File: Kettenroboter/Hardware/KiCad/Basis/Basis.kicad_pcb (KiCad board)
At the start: 2 copper layers, 90.6 x 101.2 mm, 106 parts, among them J1 691103110002, J10 691103110002, J11 Conn_01x03, J12 Conn_01x03, J13 Conn_01x03, J14 Conn_01x03, J15 Conn_01x01, J16 Conn_01x03, J17 Conn_01x03, J18 691103110002, J19 691103110002, J2 691103110002, J20 691103110002, J21 691103110002, J22 691103110002, J23 691103110002, J24 691103110002, J25 691103110002, J26 691103110002, J27 691103110002, J28 Conn_01x02, J3 691103110002, J4 691103110002, J5 691103110002, J6 691103110002, J7 691103110002, J8 691103110002, J9 691103110002, Q1 BSS138, Q2 BSS138, Q3 BSS138, Q4 BSS138, Q5 NMOS, Q6 NMOS, U2 NCP1117LPST33T3G, U3 SN74LS07

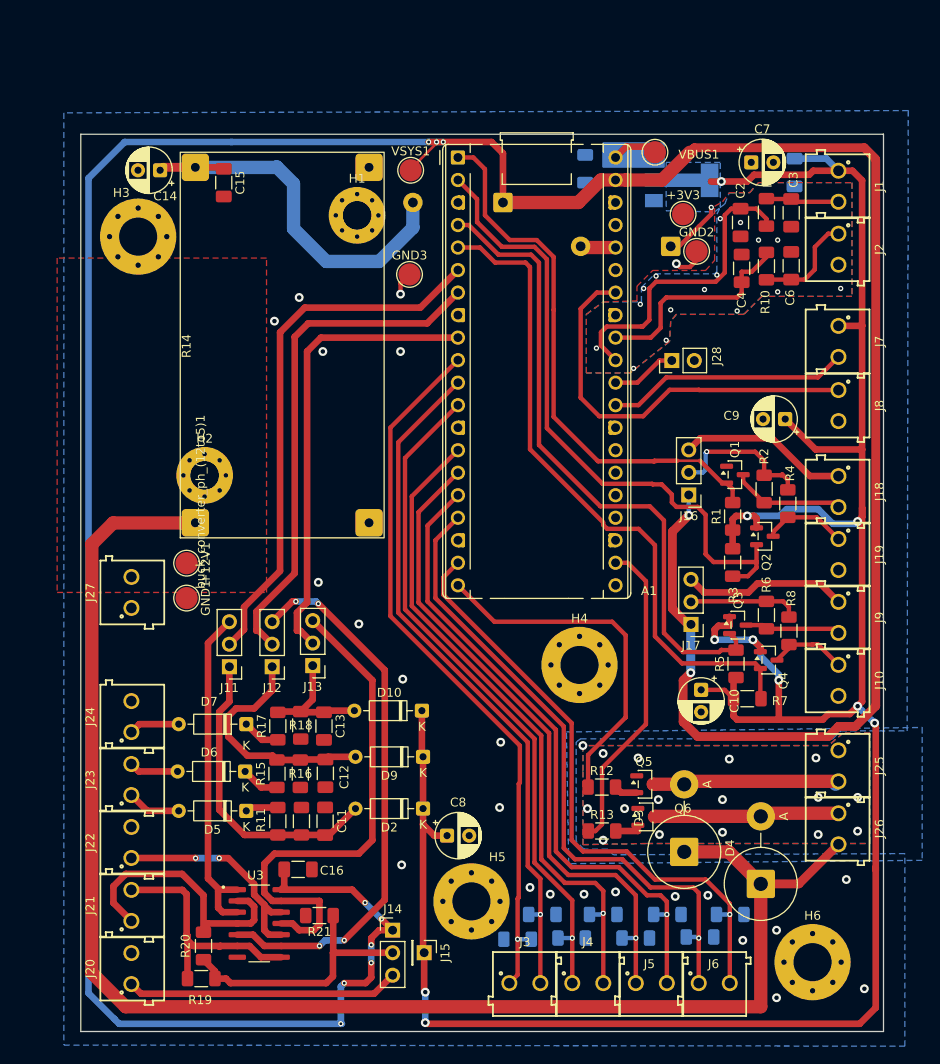
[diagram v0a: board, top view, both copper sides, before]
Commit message: final final final
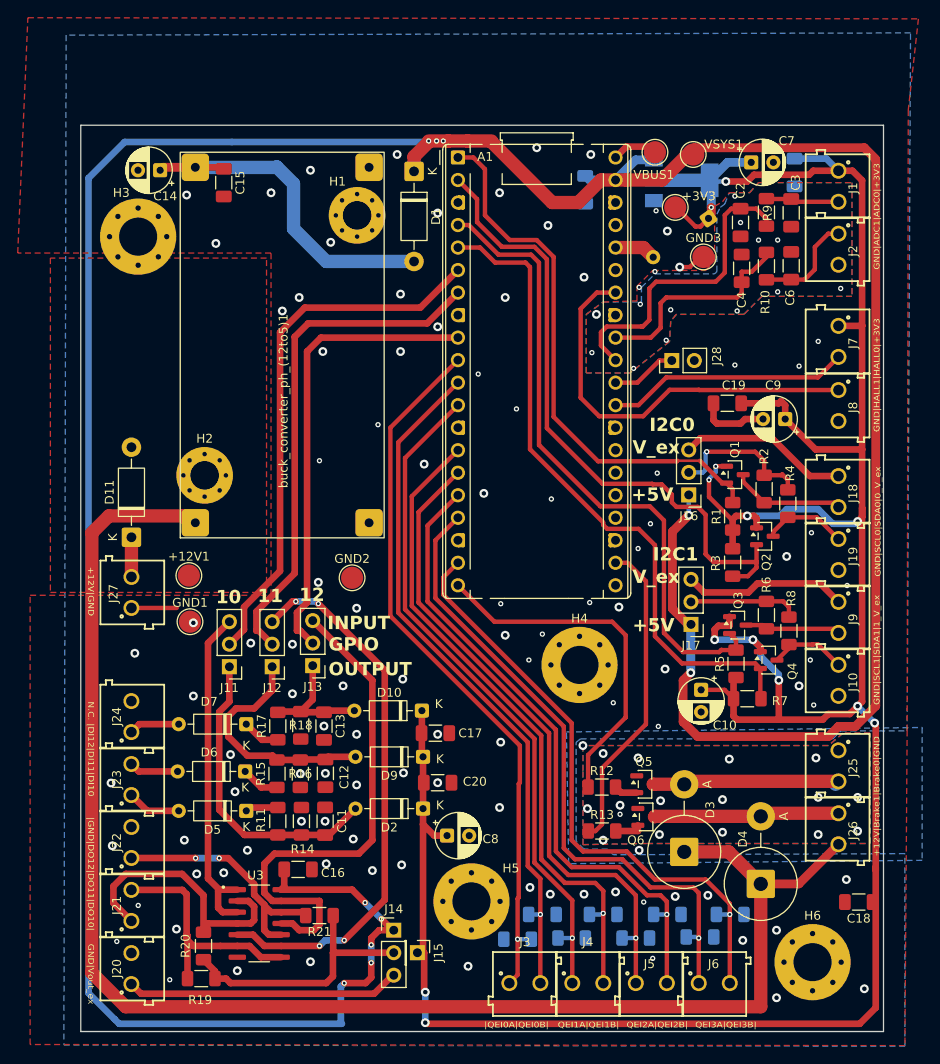
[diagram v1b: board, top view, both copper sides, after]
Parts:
- added C17: 10n, Capacitor_SMD:C_1206_3216Metric_Pad1.33x1.80mm_HandSolder, F.Cu at (127.1, 104.4)
- added C18: 10n, Capacitor_SMD:C_1206_3216Metric_Pad1.33x1.80mm_HandSolder, F.Cu at (174.9, 123.4)
- added C19: 10n, Capacitor_SMD:C_1206_3216Metric_Pad1.33x1.80mm_HandSolder, F.Cu at (160.1, 67.2)
- added C20: 10n, Capacitor_SMD:C_1206_3216Metric_Pad1.33x1.80mm_HandSolder, F.Cu at (127.4, 110.0)
- added D11: 1N5817, Diode_THT:D_DO-41_SOD81_P10.16mm_Horizontal, F.Cu at (92.8, 82.3)
- D1: moved to F.Cu
- D8: value 1N5817 -> BAT46; footprint Diode_THT:D_DO-41_SOD81_P10.16mm_Horizontal -> Diode_THT:D_DO-35_SOD27_P7.62mm_Horizontal
- moved GND2 53.5 mm to (117.7, 86.9)
- moved GND3 33.2 mm to (157.4, 50.7)
- moved VSYS1 31.9 mm to (156.2, 39.1)
- moved D1 10.6 mm to (124.7, 41.0), turned to -90 degrees
- moved D8 5.30 mm to (157.9, 46.3), turned to -145 degrees
- moved GND1 2.69 mm to (99.4, 91.8), turned to 0 degrees
- moved C1 2.36 mm to (144.0, 43.1)
- moved +12V1 1.42 mm to (99.3, 86.6), turned to 0 degrees
- moved +3V3 1.17 mm to (154.2, 45.1)
- moved J15 0.76 mm to (125.1, 129.2)
- moved J14 0.13 mm to (122.4, 126.6)
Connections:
- C1 pad 1: /VBUS -> /VSYS
- H1 pad 1: GND -> unconnected-(H1-Pad1)
- H2 pad 1: GND -> unconnected-(H2-Pad1)
- H3 pad 1: GND -> unconnected-(H3-Pad1)
- H4 pad 1: GND -> unconnected-(H4-Pad1)
- H5 pad 1: GND -> unconnected-(H5-Pad1)
- H6 pad 1: GND -> unconnected-(H6-Pad1)
- J20 pad 1: GND -> V_D_out_ext
- J20 pad 2: V_D_out_ext -> GND
- J25 pad 1: /PWR-GND -> GND
- J27 pad 2: /+12V -> Net-(D11-K)
- Q1 pad 3: I2C0 -SDA - HV -> I2C0 - SDA - HV
- Q5 pad 3: /PWR-GND -> GND
- Q6 pad 3: /PWR-GND -> GND
- R2 pad 2: I2C0 -SDA - HV -> I2C0 - SDA - HV
- U2 pad 3: /VBUS -> /VSYS
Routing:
- net /+3V3: track 300.5 -> 322.7 mm, vias 11 -> 13
- net I2C0 -SDA - HV: track 12.7 -> 0.00 mm
- net I2C0 - SDA - HV: track 0.00 -> 12.7 mm
- net GND: track 5.76 -> 15.5 mm, vias 55 -> 137
- net Net-(D11-K): track 0.00 -> 4.47 mm
- net Net-(D1-A): track 44.3 -> 40.1 mm
- net D_out_12: track 25.1 -> 28.0 mm
- net /+12V: track 172.1 -> 173.5 mm
- net /VBUS: track 6.45 -> 5.62 mm
- net Net-(A1-3V3): track 3.99 -> 4.70 mm
- net /VSYS: track 379.0 -> 378.3 mm, vias 11 -> 10
- removed copper zone on B.Cu, net /+3V3
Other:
- board size 90.6 x 101.2 mm -> 90.6 x 102.2 mm
- board text added: "+12V|Brake1|Brake0|GND"
- board text added: "+12V|GND"
- board text added: "+5V"
- board text added: "10"
- board text added: "11"
- board text added: "12"
- board text added: "GND|ADC1|ADC0|+3V3"
- board text added: "GND|HALL1|HALL0|+3V3"
- board text added: "GND|SCL0|SDA0|0_V_ex"
- board text added: "GND|SCL1|SDA1|1_V_ex"
- board text added: "GND|Vout_ex"
- board text added: "GPIO"
- board text added: "I2C0"
- board text added: "I2C1"
- board text added: "INPUT"
- board text added: "N.C. |DI12|DI11|DI10"
- board text added: "OUTPUT"
- board text added: "QEI1A|QEI1B|"
- board text added: "QEI2A|QEI2B|"
- board text added: "QEI3A|QEI3B|"
- board text added: "V_ex"
- board text added: "|GND|DO12|DO11|DO10|"
- board text added: "|QEI0A|QEI0B|"
